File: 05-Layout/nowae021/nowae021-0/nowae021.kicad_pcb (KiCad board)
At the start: 2 copper layers, 25.4 x 25.4 mm, 37 parts, among them P1 NVT_BUS, P2 NVT_BUS, Q1 PDTC123EU, Q2 PDTC123EU, Q3 PDTC123EU, Q4 PDTC123EU, Q5 PDTC123EU, Q6 PDTC123EU, SW1 BUTTON-WE_434153017835, U1 MKL15Z128VFM4, U2 TPS70933DBV, Y1 32768

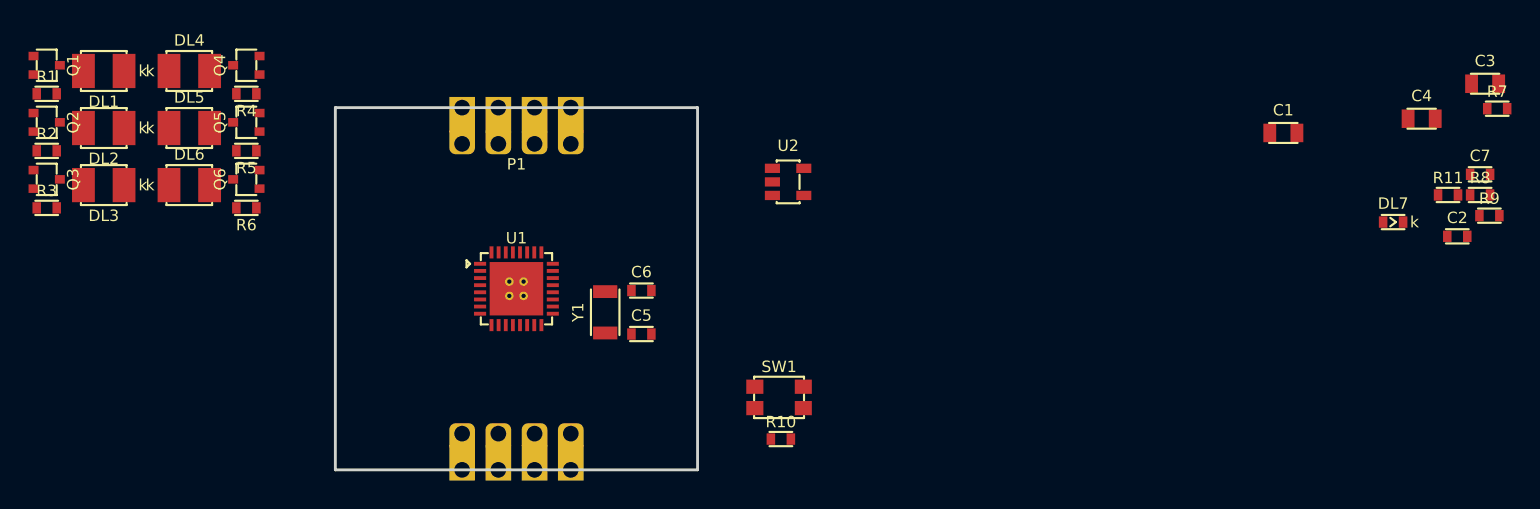
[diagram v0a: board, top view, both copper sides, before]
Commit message: WiP routing (nowae021-0)
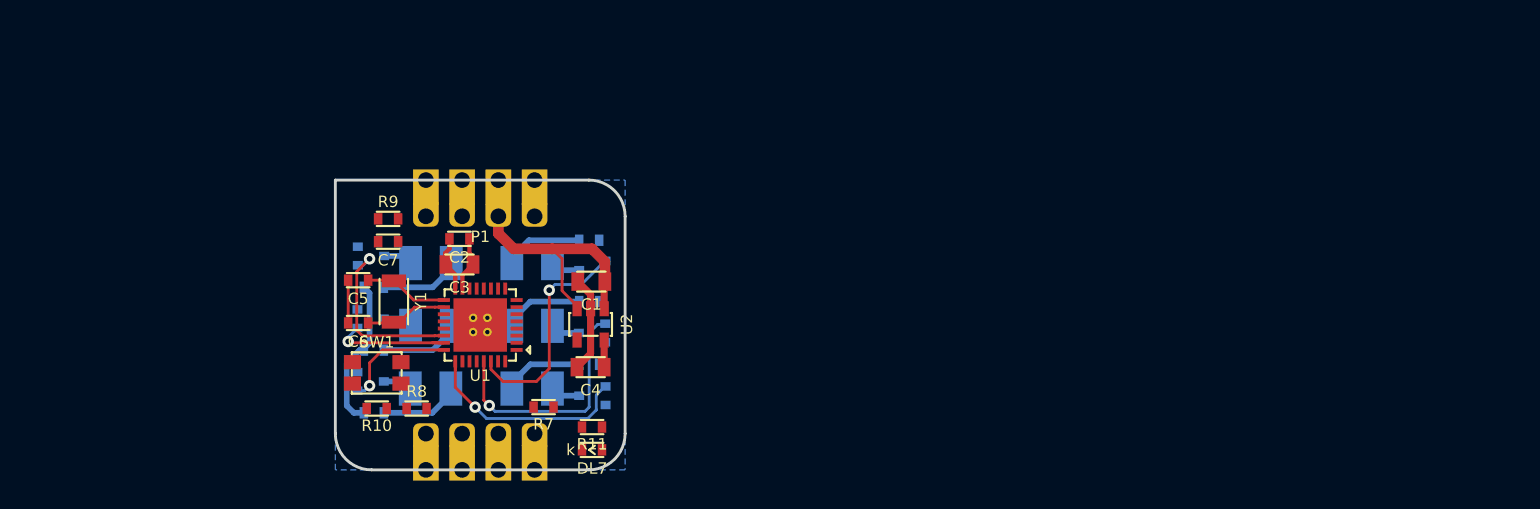
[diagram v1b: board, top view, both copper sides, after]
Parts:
- DL1, DL2, DL3, DL4, DL5, DL6, Q1, Q2, Q3, Q4, Q5, Q6, R1, R2, R3, R4, R5, R6: moved to B.Cu
- moved R9 77.2 mm to (105.7, 73.4)
- moved C7 76.7 mm to (105.7, 75.0), turned to 180 degrees
- moved R8 76.1 mm to (107.7, 86.7)
- moved C3 73.0 mm to (110.7, 76.6), turned to 180 degrees
- moved R7 70.1 mm to (116.6, 86.6), turned to 180 degrees
- moved C2 70.0 mm to (110.7, 74.8), turned to 180 degrees
- moved R11 62.2 mm to (120.0, 88.0), turned to 180 degrees
- moved C4 60.8 mm to (119.9, 83.8), turned to 180 degrees
- moved DL7 58.4 mm to (120.0, 89.6), turned to 180 degrees
- moved C1 49.6 mm to (120.0, 77.8), turned to 180 degrees
- moved Q6 28.6 mm to (120.0, 85.8), turned to 270 degrees
- moved R10 28.4 mm to (104.9, 86.7), turned to 180 degrees
- moved Q5 28.4 mm to (120.0, 81.4), turned to 270 degrees
- moved SW1 28.3 mm to (104.9, 84.2)
- moved Q4 28.2 mm to (120.0, 77.0), turned to 270 degrees
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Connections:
- U1 pad 25: /FIRE_LED4 -> /FIRE_LED6
- U1 pad 30: /FIRE_LED6 -> /FIRE_LED4
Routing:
- net +VIN: track 0.00 -> 28.5 mm
- net /FIRE_LED5: track 0.00 -> 17.7 mm, vias 0 -> 1
- net /FIRE_LED4: track 0.00 -> 15.8 mm, vias 0 -> 1
- net /FIRE_LED6: track 0.00 -> 15.7 mm, vias 0 -> 1
- net GND: track 0.00 -> 14.1 mm
- net /FIRE_LED1: track 0.00 -> 12.7 mm, vias 0 -> 1
- net /FIRE_LED2: track 0.00 -> 8.78 mm, vias 0 -> 1
- net /FIRE_LED3: track 0.00 -> 8.18 mm, vias 0 -> 1
- net Net-(C5-Pad1): track 0.00 -> 5.89 mm
- net +3.3V: track 0.00 -> 5.80 mm
- net Net-(C6-Pad1): track 0.00 -> 5.77 mm
- net Net-(DL5-Pad1): track 0.00 -> 5.66 mm
- net Net-(DL1-Pad1): track 0.00 -> 5.66 mm
- net Net-(DL6-Pad1): track 0.00 -> 5.66 mm
- net Net-(DL2-Pad1): track 0.00 -> 5.66 mm
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- added copper zone on B.Cu, net GND
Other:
- board size 25.4 x 25.4 mm -> 20.3 x 20.3 mm
- net class Default: trace_width 0.25 -> 0.2
- rule via_min_size: 0.4 -> 0.6
